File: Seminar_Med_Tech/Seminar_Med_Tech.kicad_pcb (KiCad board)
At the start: 2 copper layers, 96 x 88 mm, 160 parts, among them J1 CONN_02X08, J3 CONN_02X10, J5 CONN_02X10, J7 CONN_02X08, U1 OPA132, U18 ADS1298, U20 ADS1298, U4 LM317T, U5 LM317T, U6 LM337K

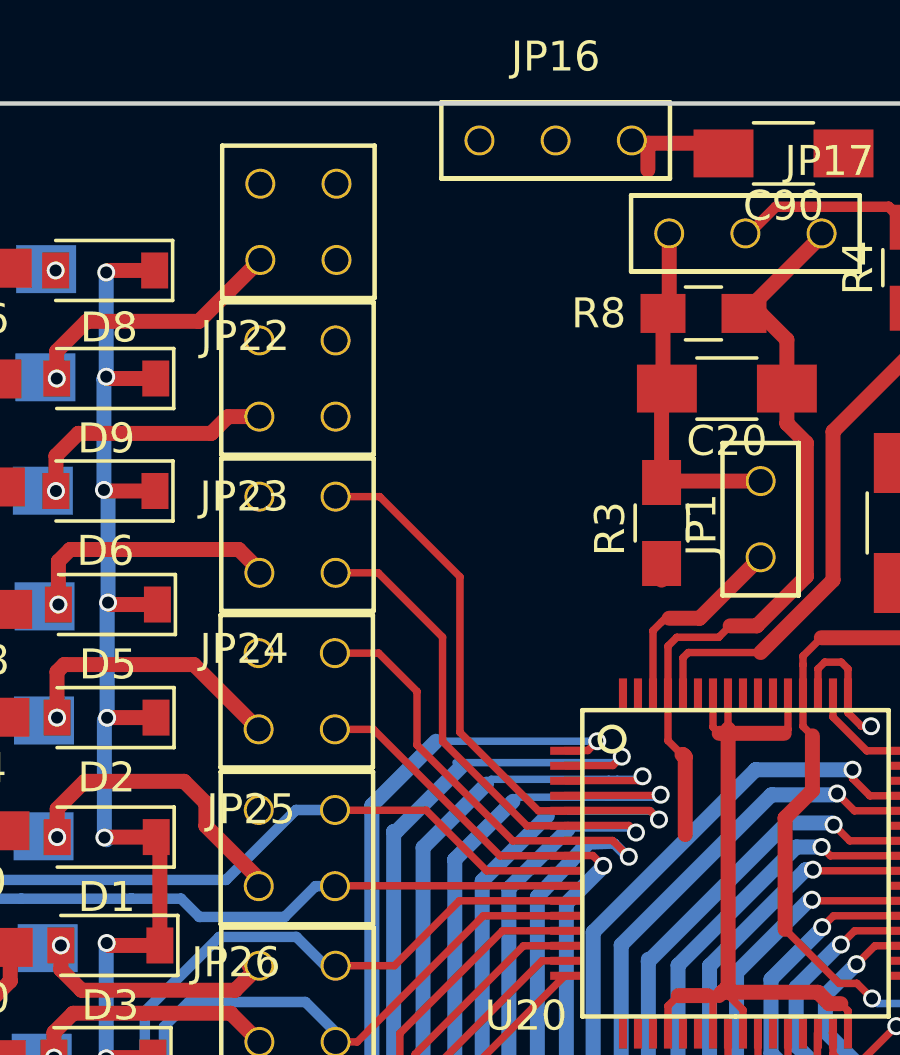
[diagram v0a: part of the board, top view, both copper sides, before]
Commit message: Update
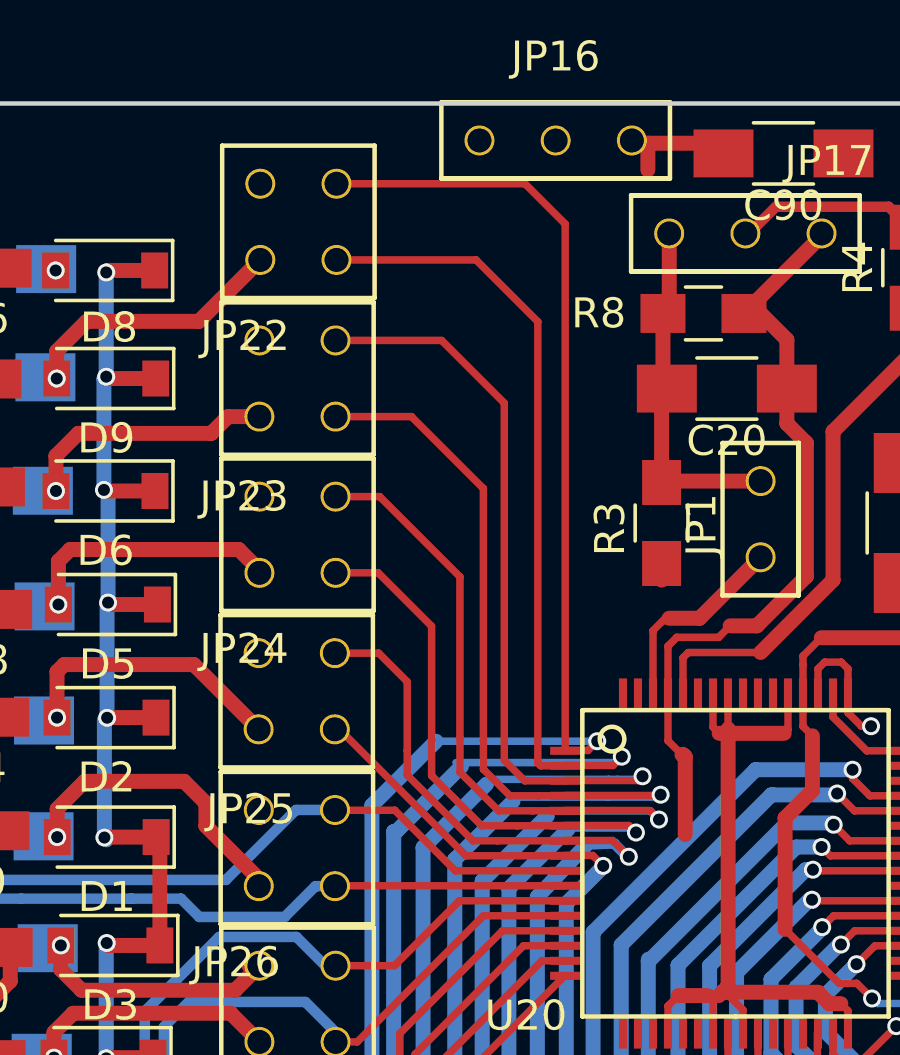
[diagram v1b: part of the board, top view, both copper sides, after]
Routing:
- net ECG_8N: track 50.1 -> 75.8 mm
- net ECG_8P: track 53.4 -> 76.6 mm
- net ECG_7N: track 49.6 -> 70.3 mm
- net ECG_7P: track 52.3 -> 70.7 mm
- net ECG_6P: track 60.5 -> 61.4 mm
- net ECG_5N: track 53.5 -> 54.3 mm
- net ECG_6N: track 62.4 -> 63.1 mm
